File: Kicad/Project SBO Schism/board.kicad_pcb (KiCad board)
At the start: 2 copper layers, 122.3 x 118.1 mm, 50 parts

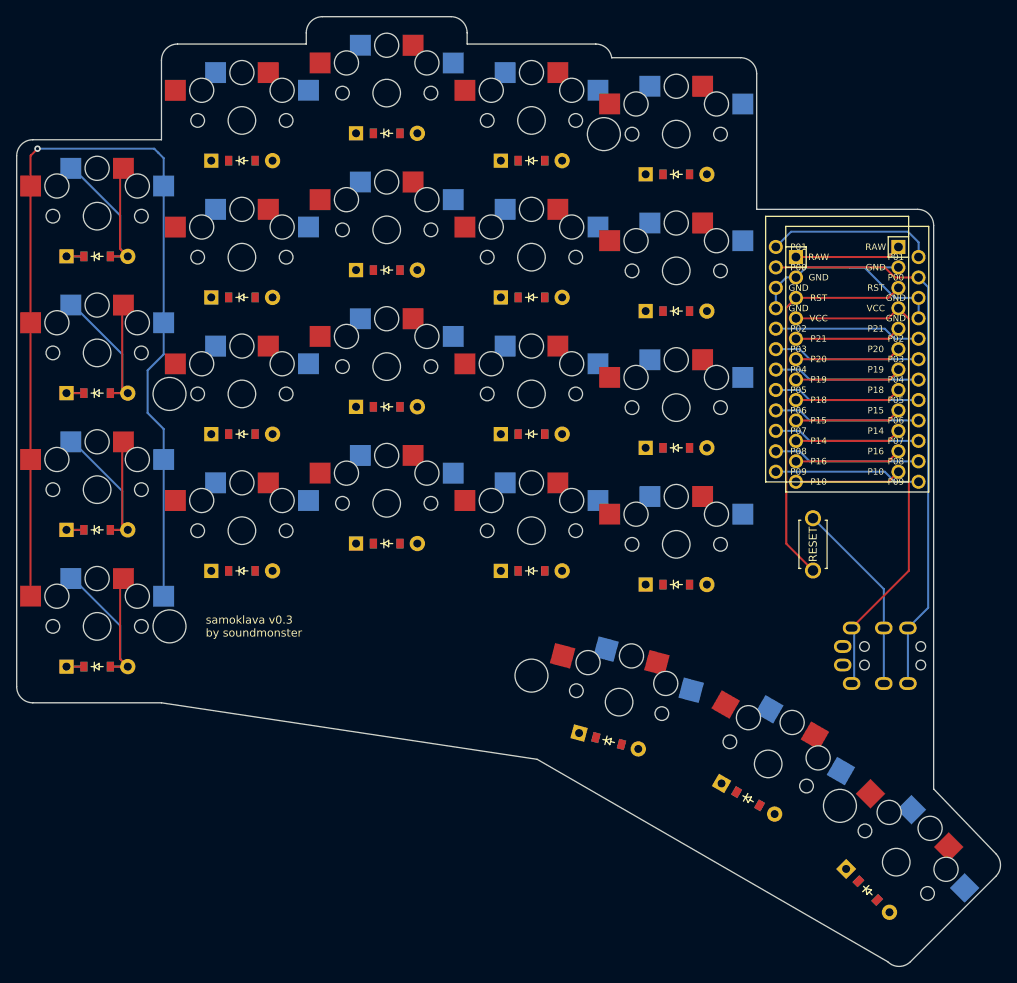
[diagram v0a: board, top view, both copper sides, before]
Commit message: Work continues
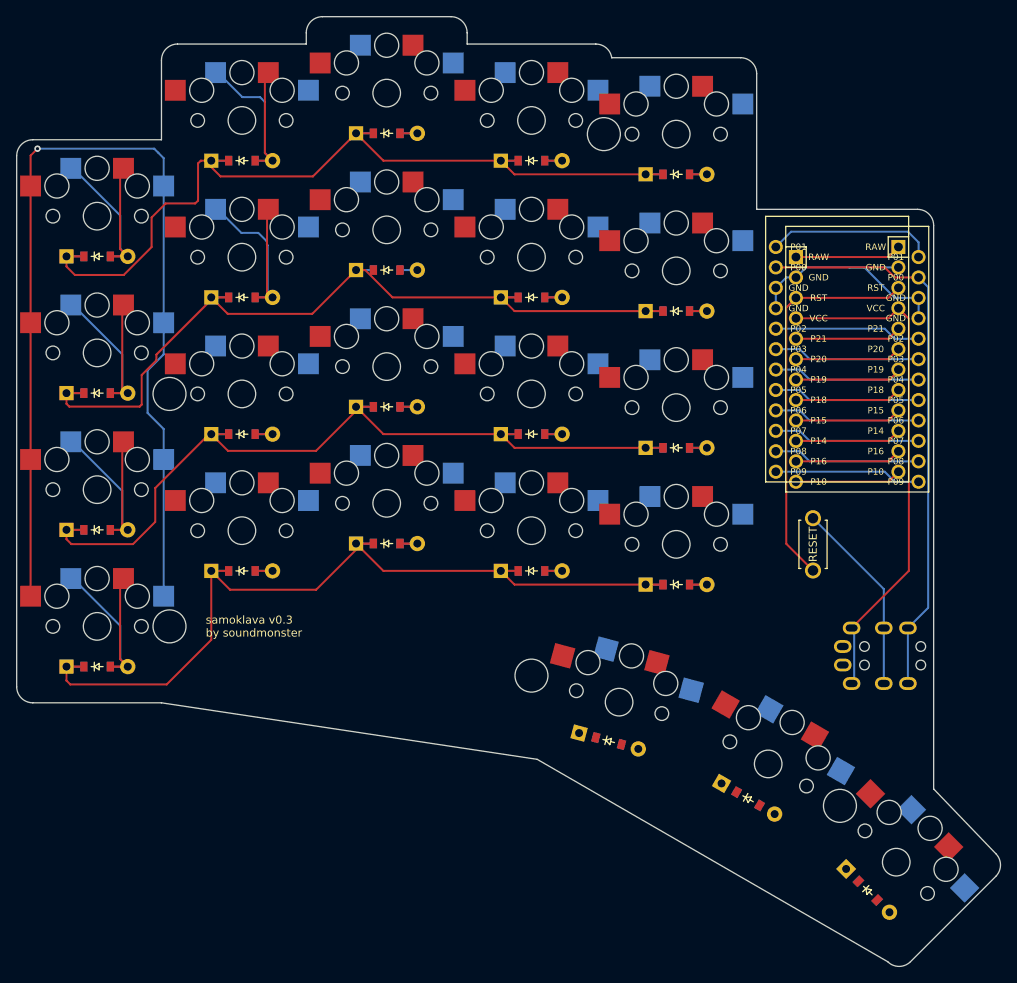
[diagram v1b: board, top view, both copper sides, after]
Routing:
- net row_bottom: track 22.6 -> 130.6 mm
- net row_extra: track 22.6 -> 129.9 mm
- net row_home: track 22.6 -> 126.9 mm
- net row_top: track 22.6 -> 124.8 mm
- net ring_extra: track 0.00 -> 31.2 mm
- net ring_top: track 0.00 -> 30.9 mm
- net middle_home: track 0.00 -> 4.32 mm
- net middle_extra: track 0.00 -> 4.32 mm
- net middle_bottom: track 0.00 -> 4.32 mm
- net index_top: track 0.00 -> 4.32 mm
- net index_home: track 0.00 -> 4.32 mm
- net index_extra: track 0.00 -> 4.32 mm
- net index_bottom: track 0.00 -> 4.32 mm
- net ring_home: track 0.00 -> 4.32 mm
- net ring_bottom: track 0.00 -> 4.32 mm
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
